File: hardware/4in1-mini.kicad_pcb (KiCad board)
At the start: 6 copper layers, 31.2 x 33 mm, 186 parts, among them J1 SM08B-SRSS-TB, Q1 DOY180N03T, Q10 DOY180N03T, Q11 DOY180N03T, Q12 DOY180N03T, Q13 DOY180N03T, Q14 DOY180N03T, Q15 DOY180N03T, Q16 DOY180N03T, Q17 DOY180N03T, Q18 DOY180N03T, Q19 DOY180N03T, Q2 DOY180N03T, Q20 DOY180N03T, Q21 DOY180N03T, Q22 DOY180N03T, Q23 DOY180N03T, Q24 DOY180N03T, Q3 DOY180N03T, Q4 DOY180N03T, Q5 DOY180N03T, Q6 DOY180N03T, Q7 DOY180N03T, Q8 DOY180N03T, Q9 DOY180N03T, U1 TLV76733DRVR, U10 AT32F421G8U7, U11 NSG2065Q, U12 INA186A3IDCKR, U13 LMR54406DBVR, U2 AT32F421G8U7, U3 NSG2065Q, U5 FTC160808S4R7MBCA, U6 AT32F421G8U7, U7 NSG2065Q, U8 AT32F421G8U7, U9 NSG2065Q

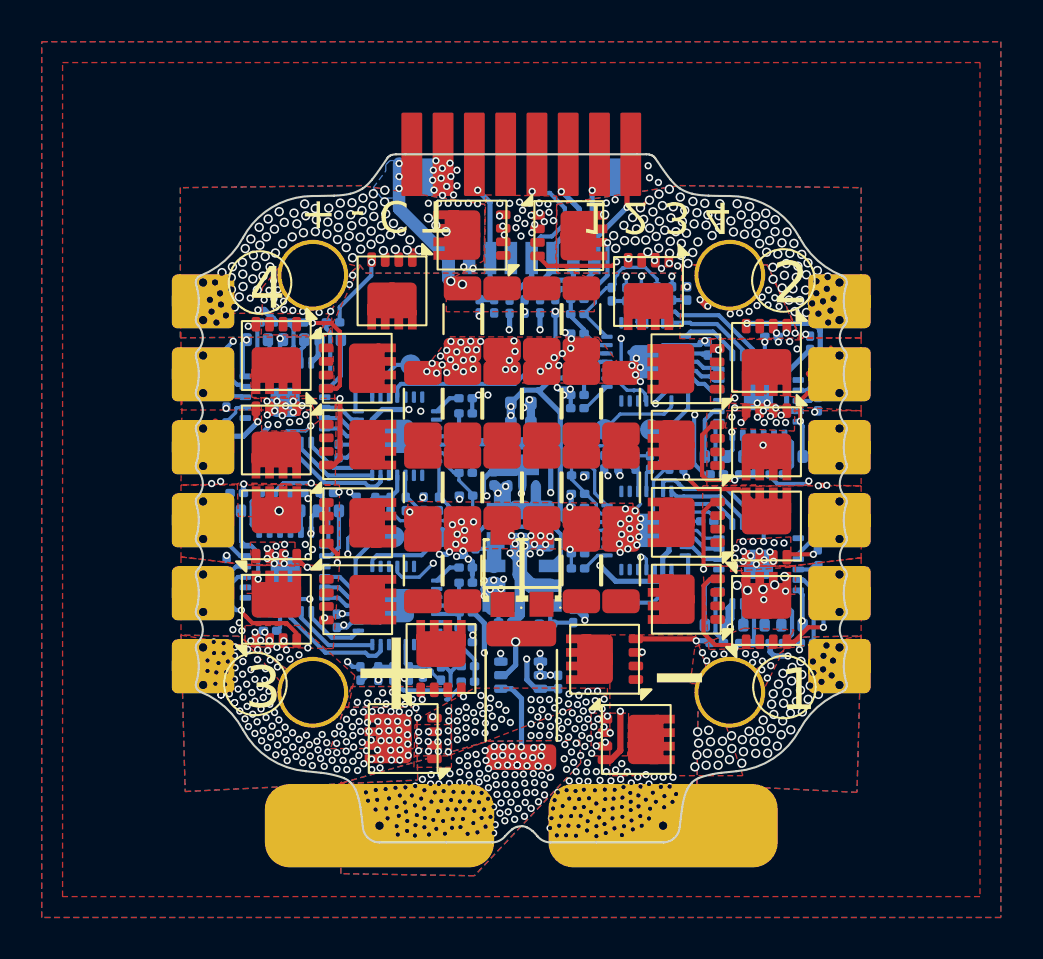
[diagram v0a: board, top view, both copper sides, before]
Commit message: SFT naming update
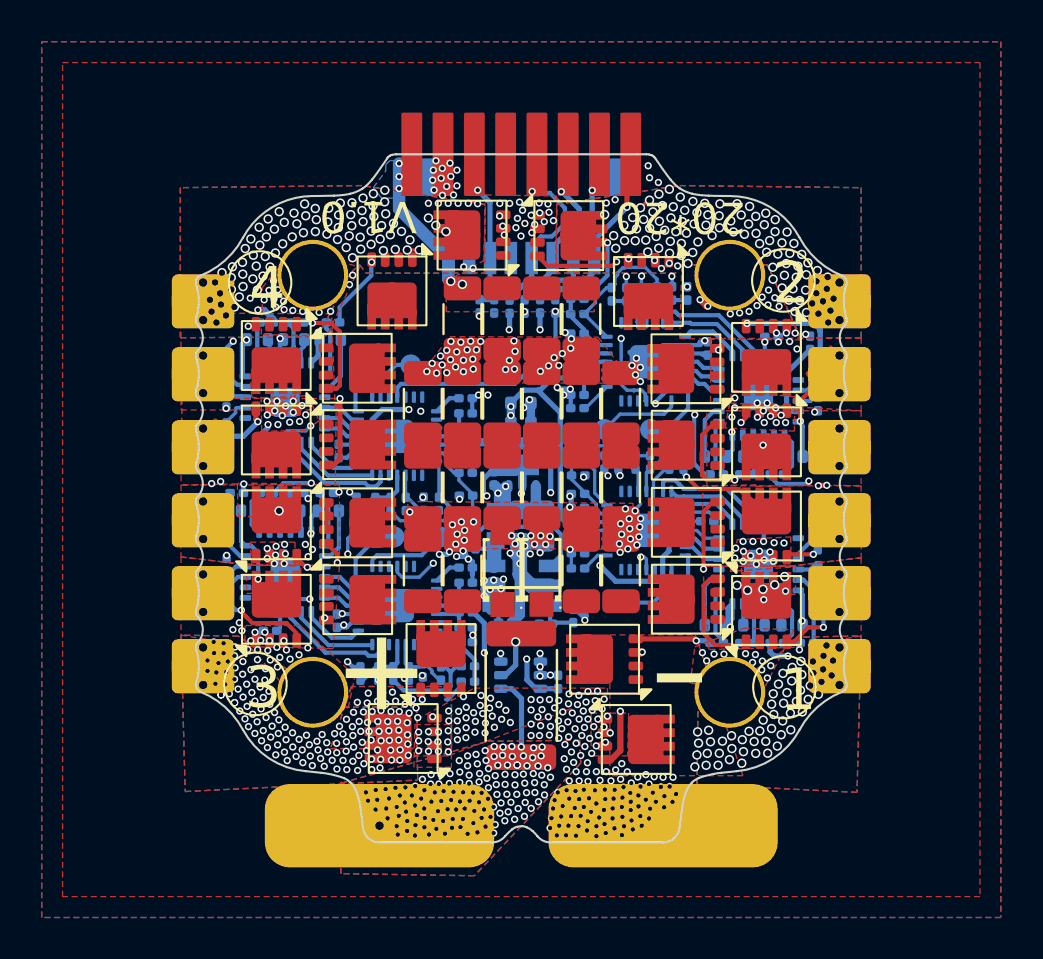
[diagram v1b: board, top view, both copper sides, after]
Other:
- board text added: "20*20"
- board text added: "FPV"
- board text added: "Shadow"
- board text added: "V1.0"
- board text removed: "+ - C T"
- board text removed: "1 2 3 4"
- board text removed: "AM32"
- board text removed: "ESC"
- board text removed: "open"
